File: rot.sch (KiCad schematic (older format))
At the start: 34 parts, among them J3 543630489, J4 M20-7830642, U2 W25Q32JVSSIQ_TR, U3 W25Q32JVSSIQ_TR, U4 W25Q32JVSSIQ_TR, U5 W25Q32JVSSIQ_TR

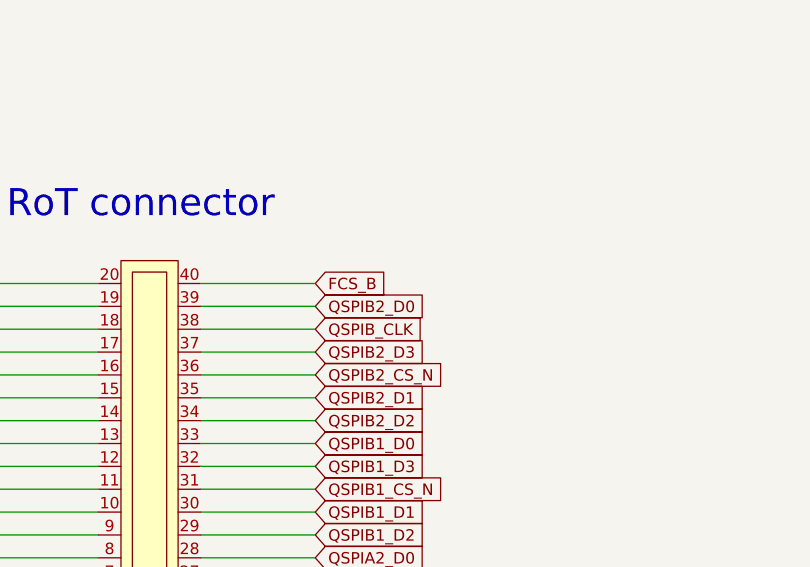
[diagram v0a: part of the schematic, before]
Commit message: Added local libs
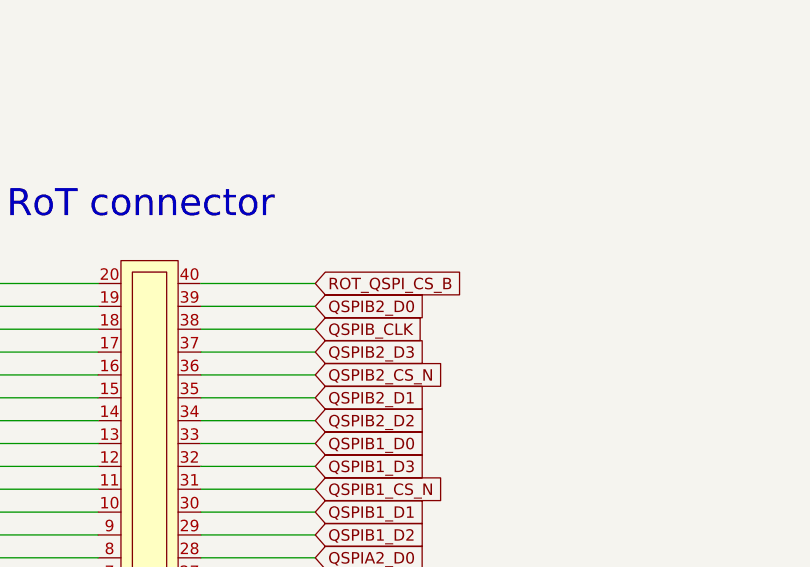
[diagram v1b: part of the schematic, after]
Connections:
- net FCS_B renamed ROT_QSPI_CS_B
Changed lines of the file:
@@
 	1    0    0    1
 $EndComp
-Text GLabel 9675 4625 2    50   Input ~ 0
-FCS_B
 Text GLabel 8225 5325 0    50   Input ~ 0
 ROT_QSPI_SCK
@@
 	1    0    0    -1
 $EndComp
+Text GLabel 9675 4625 2    50   Input ~ 0
+ROT_QSPI_CS_B
 $EndSCHEMATC
